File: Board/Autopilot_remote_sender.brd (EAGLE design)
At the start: 24 parts

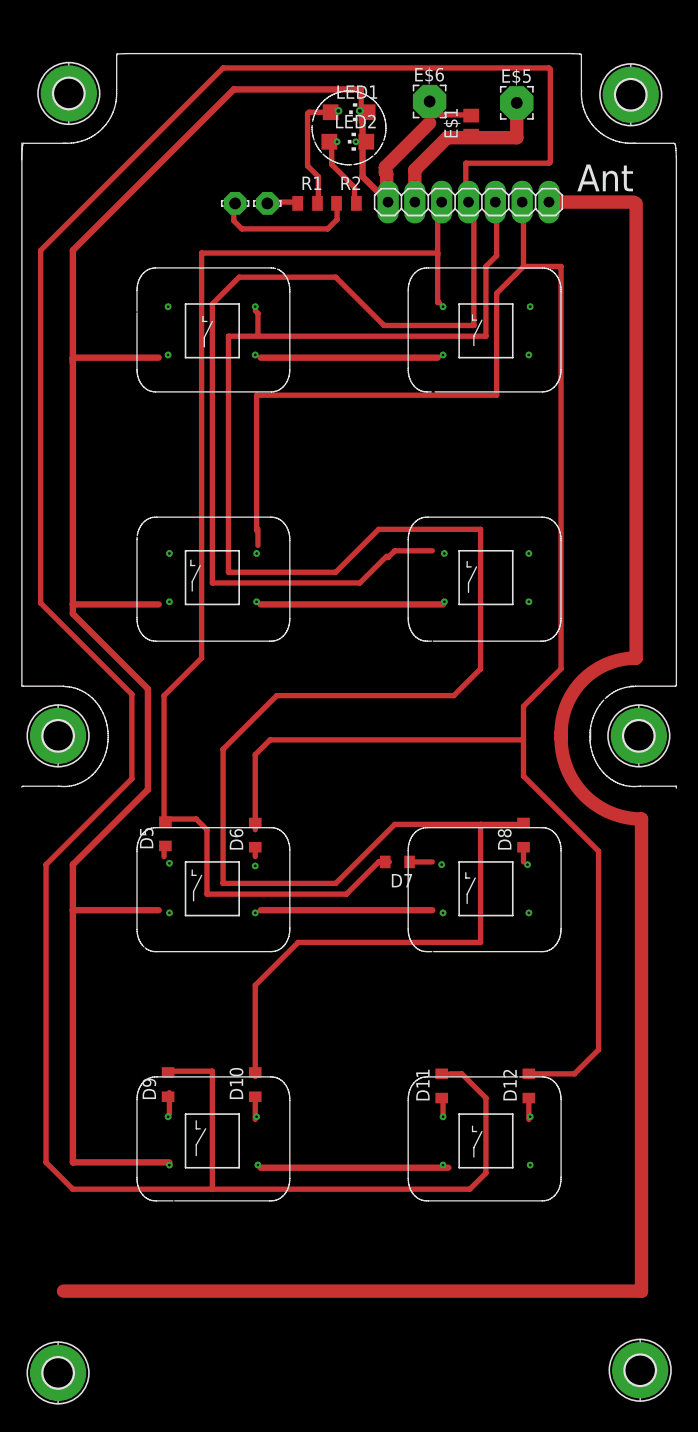
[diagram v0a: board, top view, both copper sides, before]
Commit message: Add gerber files
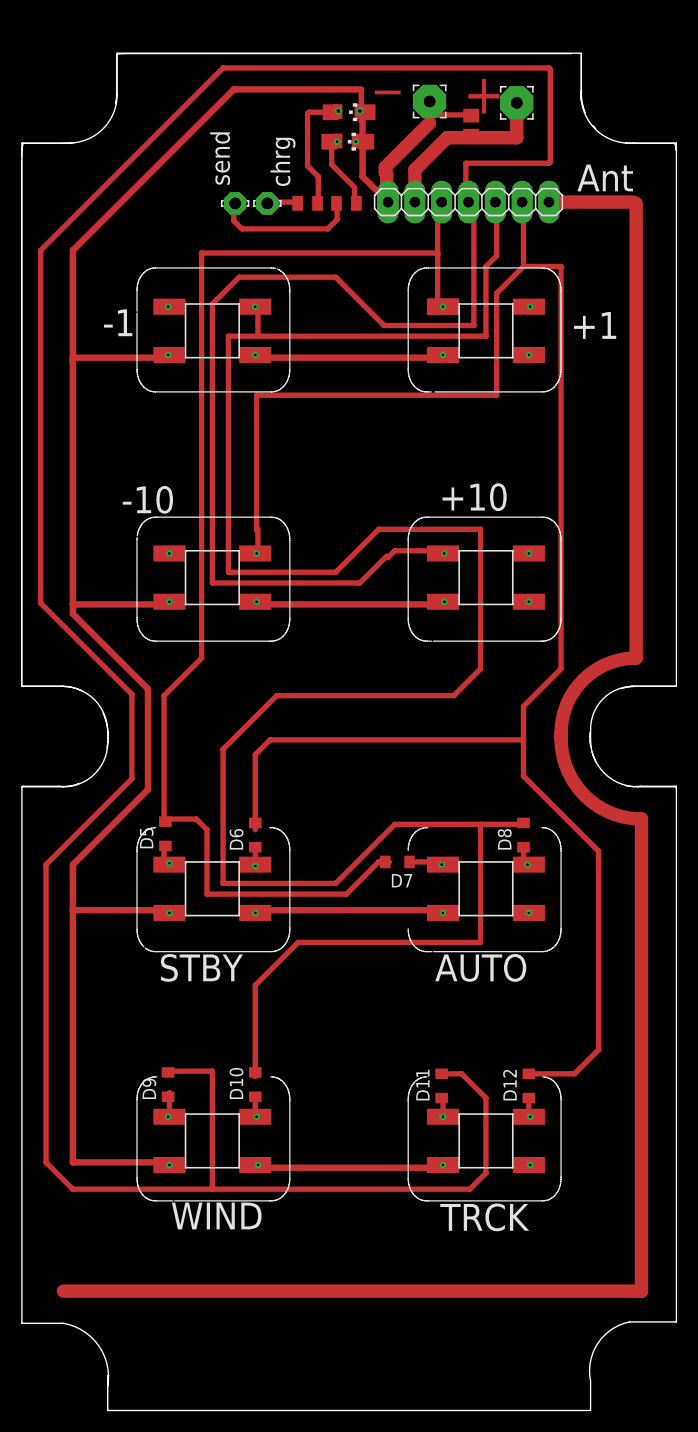
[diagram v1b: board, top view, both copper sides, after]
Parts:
- removed E$17, E$18, E$22, E$23, E$24, E$25: (no value), holes:2,8-PAD
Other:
- board outline added: 62 x 128.5 mm
